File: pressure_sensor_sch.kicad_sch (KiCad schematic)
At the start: 36 parts, among them IC5 ADS131M03IRUKR, J13 1053131104

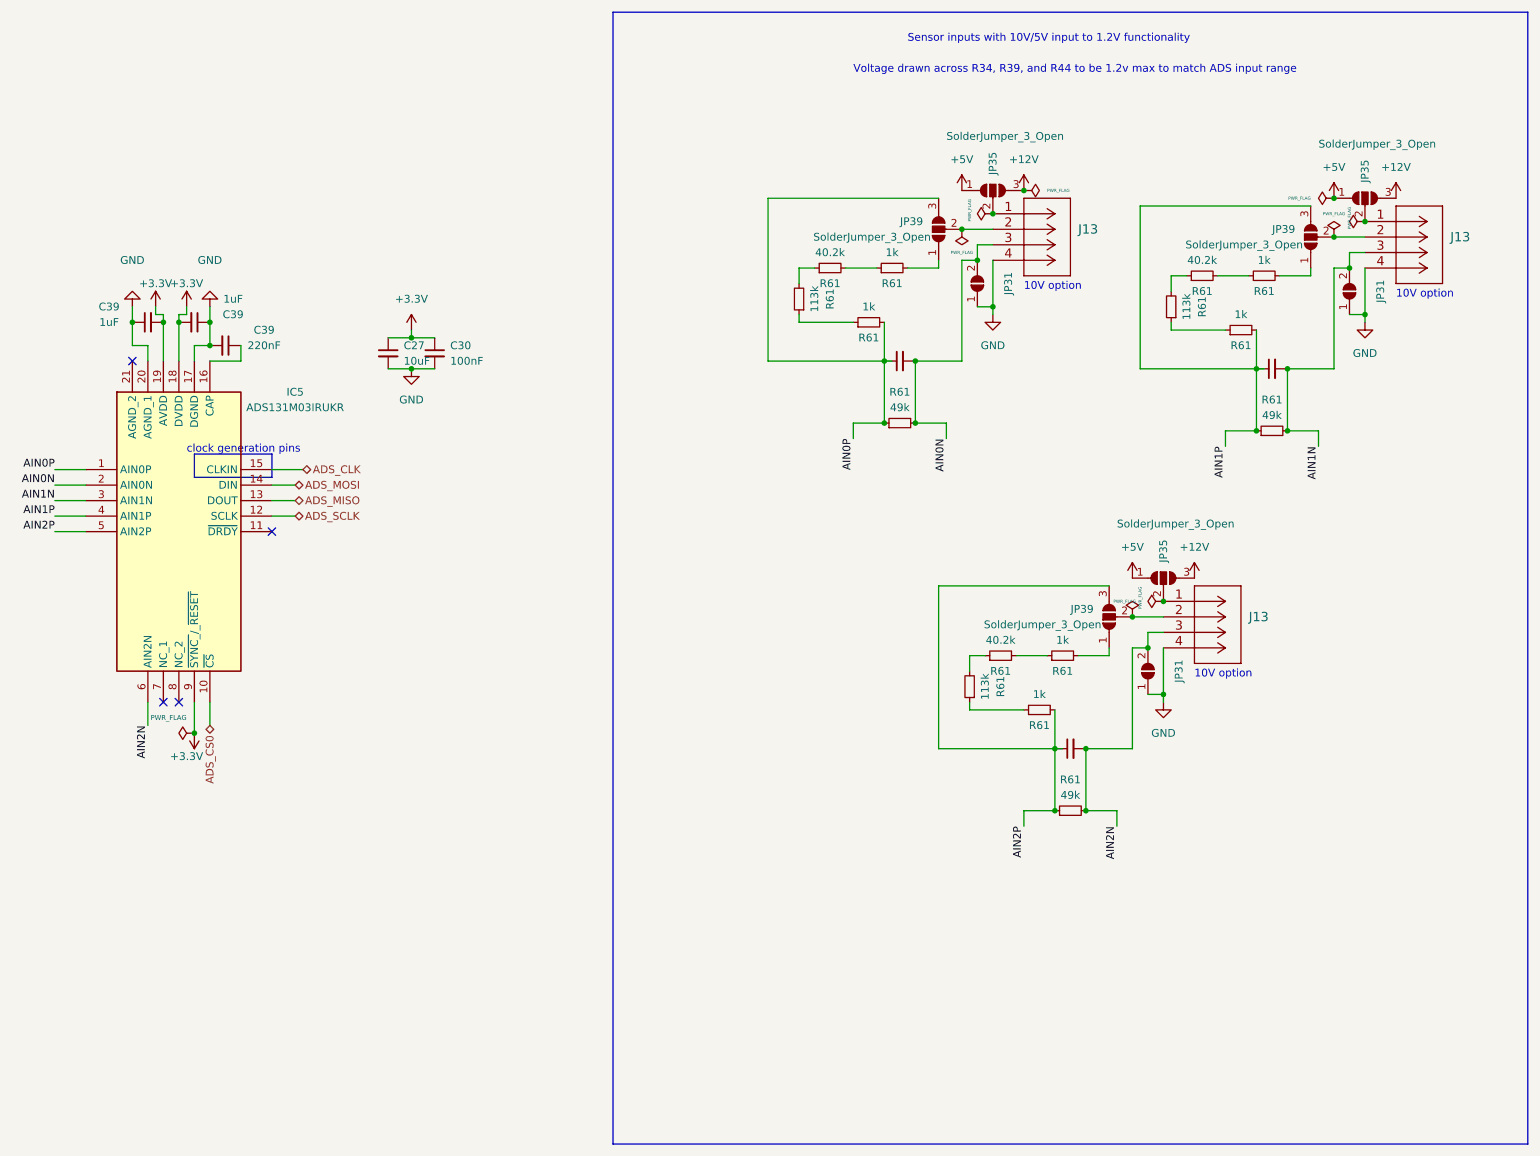
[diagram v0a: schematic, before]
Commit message: Finished schematic
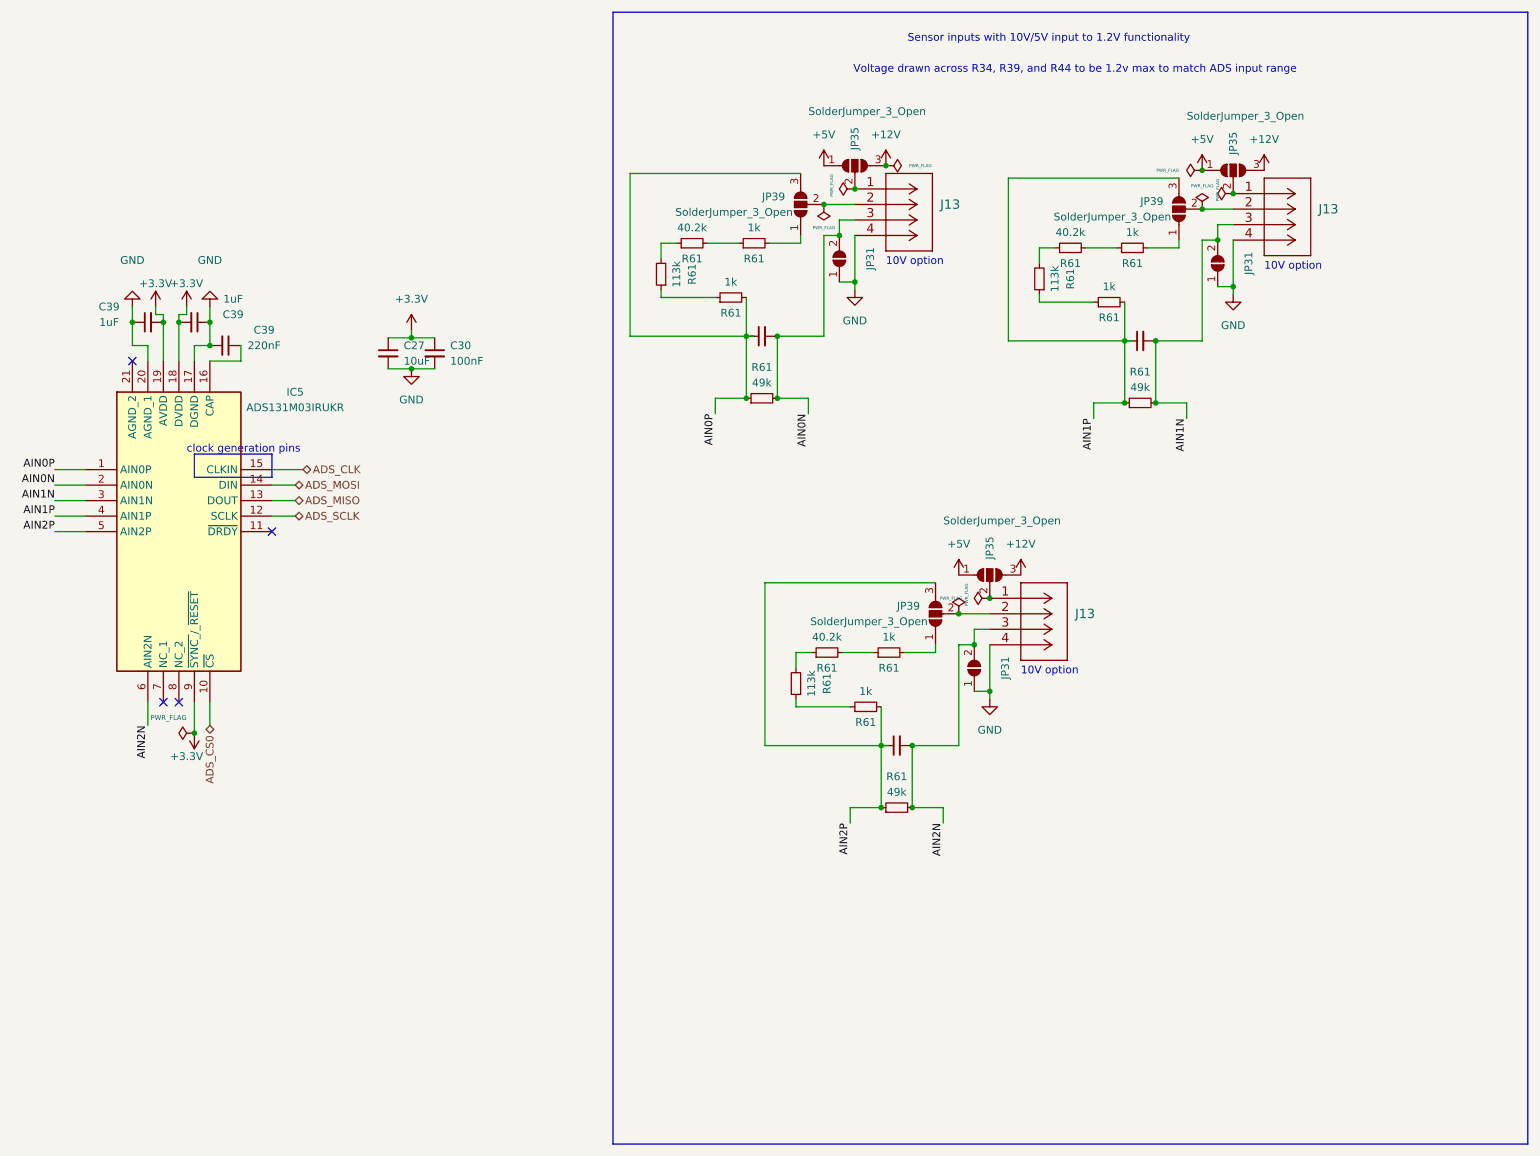
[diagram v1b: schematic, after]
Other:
- moved on the sheet: J13, JP31, JP35, JP39, R61
